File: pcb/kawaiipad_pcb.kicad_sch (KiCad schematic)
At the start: 21 parts, among them SW1 SW_Push_45deg, SW2 SW_Push_45deg, SW3 SW_Push_45deg, SW4 SW_Push_45deg, SW5 SW_Push_45deg, SW6 SW_Push_45deg, SW7 SW_Push_45deg, SW8 SW_Push_45deg, SW9 SW_Push_45deg, U1 XIAO-RP2040-DIP

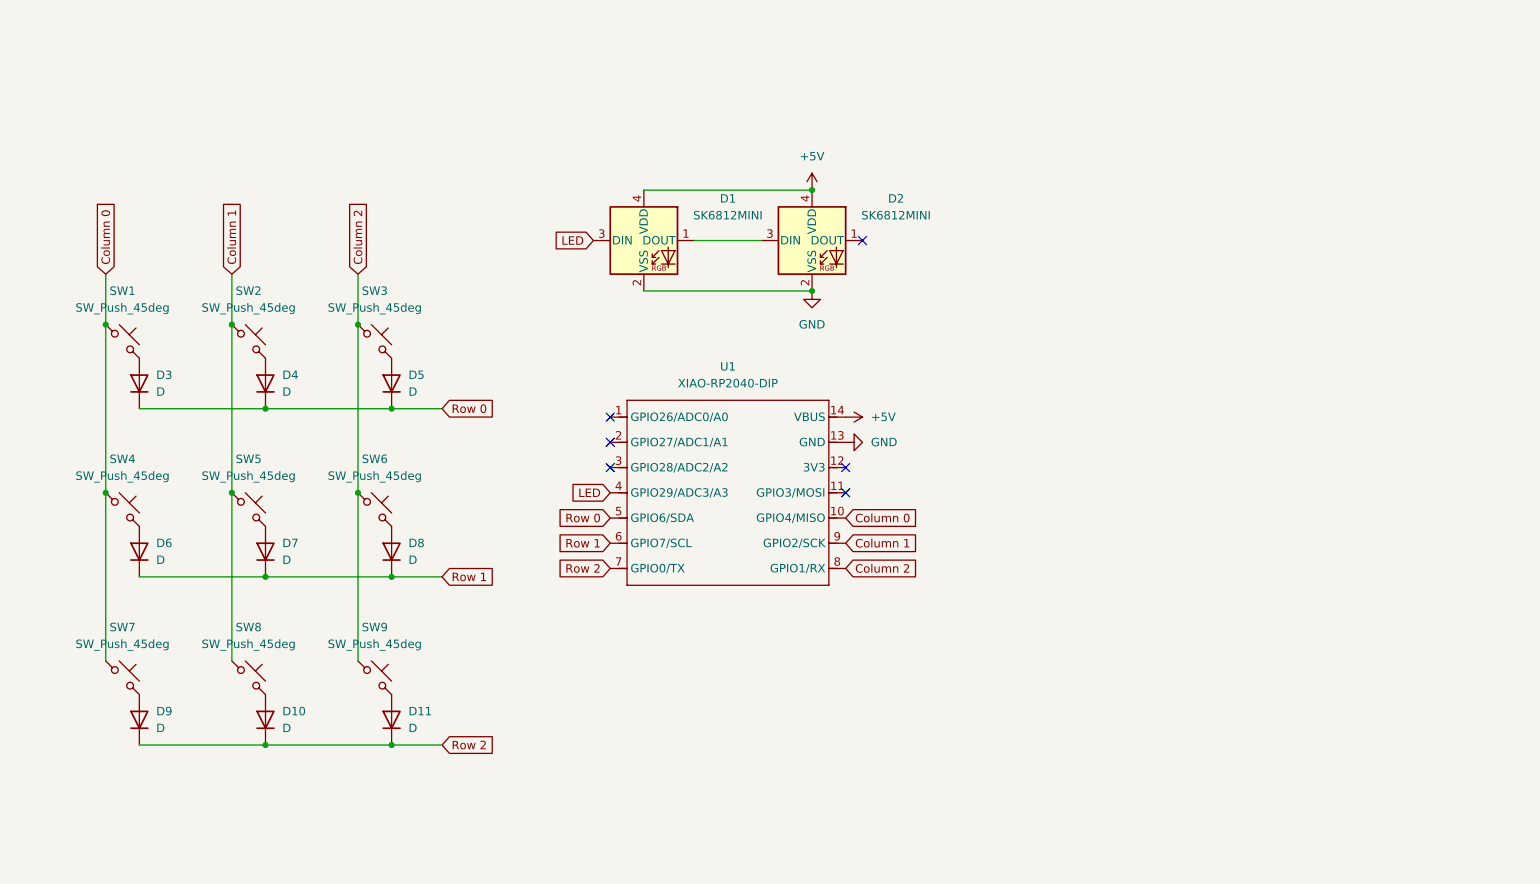
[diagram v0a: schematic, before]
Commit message: Update kawaiipad_pcb.kicad_sch
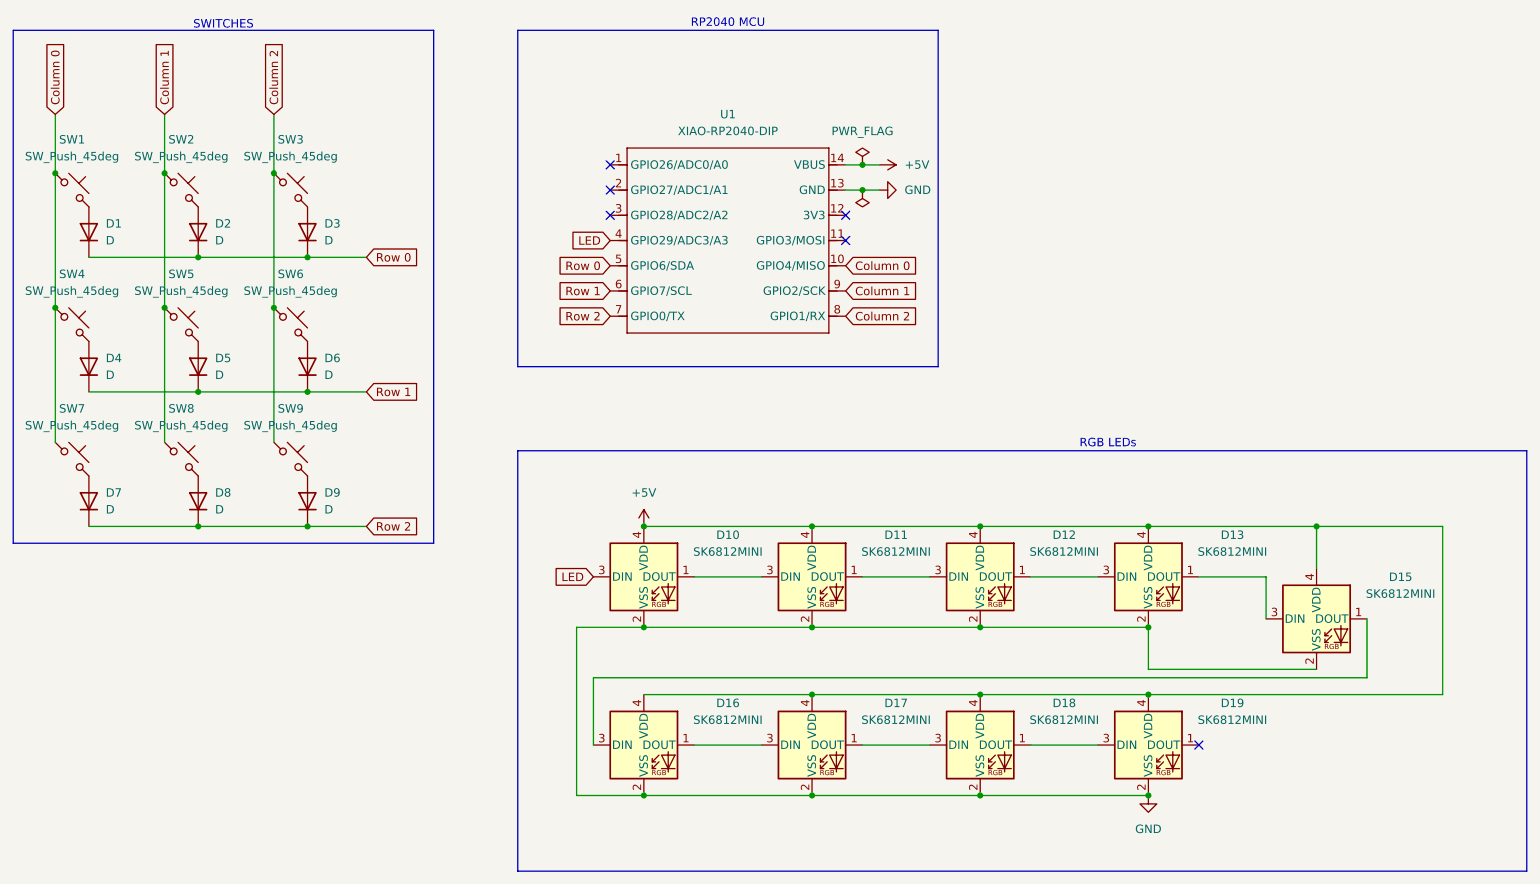
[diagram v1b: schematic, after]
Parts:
- removed D1, D2: SK6812MINI, LED_SMD:LED_SK6812MINI_PLCC4_3.5x3.5mm_P1.75mm, symbol LED:SK6812MINI
- removed D10, D11: D, DiodeLibrary:Diode-Hybrid-Dual, symbol Device:D
- added D1, D2: D, symbol Device:D
- added D10, D11, D12, D13, D15, D16, D17, D18, D19: SK6812MINI, LED_SMD:LED_SK6812MINI_PLCC4_3.5x3.5mm_P1.75mm, symbol LED:SK6812MINI
- D3, D4, D5, D6, D7, D8, D9: footprint DiodeLibrary:Diode-Hybrid-Dual -> (none)
- SW1, SW2, SW3, SW4, SW5, SW6, SW7, SW8, SW9: footprint Button_Switch_Keyboard:SW_Cherry_MX_1.00u_PCB -> (none)
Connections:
- net +5V: now also D10.4 (VDD), D11.4 (VDD), D12.4 (VDD), D13.4 (VDD), D15.4 (VDD), D16.4 (VDD), D17.4 (VDD), D18.4 (VDD), D19.4 (VDD)
- net GND: now also D10.2 (VSS), D11.2 (VSS), D12.2 (VSS), D13.2 (VSS), D15.2 (VSS), D16.2 (VSS), D17.2 (VSS), D18.2 (VSS), D19.2 (VSS)
- net LED: now also D10.3 (DIN)
- net Row 0: now also D1.1 (K), D2.1 (K); no longer D4.1 (K), D5.1 (K)
- net Row 1: now also D4.1 (K), D5.1 (K); no longer D7.1 (K), D8.1 (K)
- net Row 2: now also D7.1 (K), D8.1 (K)
- net at SW8.2: now also D8.2 (A)
- net at D9.2 (A): now also SW9.2; no longer SW7.2
- net at SW6.2: now also D6.2 (A); no longer D8.2 (A)
- net at SW5.2: now also D5.2 (A); no longer D7.2 (A)
- net at SW4.2: now also D4.2 (A); no longer D6.2 (A)
- net at SW1.2: now also D1.2 (A); no longer D3.2 (A)
- net at SW3.2: now also D3.2 (A); no longer D5.2 (A)
- net at SW2.2: now also D2.2 (A); no longer D4.2 (A)
- new net: D10.1 (DOUT), D11.3 (DIN)
- new net: D11.1 (DOUT), D12.3 (DIN)
- new net: D16.1 (DOUT), D17.3 (DIN)
- new net: D15.1 (DOUT), D16.3 (DIN)
- new net: D7.2 (A), SW7.2
- new net: D12.1 (DOUT), D13.3 (DIN)
- new net: D13.1 (DOUT), D15.3 (DIN)
- new net: D18.1 (DOUT), D19.3 (DIN)
- new net: D17.1 (DOUT), D18.3 (DIN)
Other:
- note added: "RGB LEDs"
- note added: "RP2040 MCU"
- note added: "SWITCHES"
- title: (none) -> KawaiiPad
- moved on the sheet: U1
